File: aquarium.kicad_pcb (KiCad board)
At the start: 2 copper layers, 104 x 47 mm, 40 parts, among them U1 MOC3063, U2 MOC3063

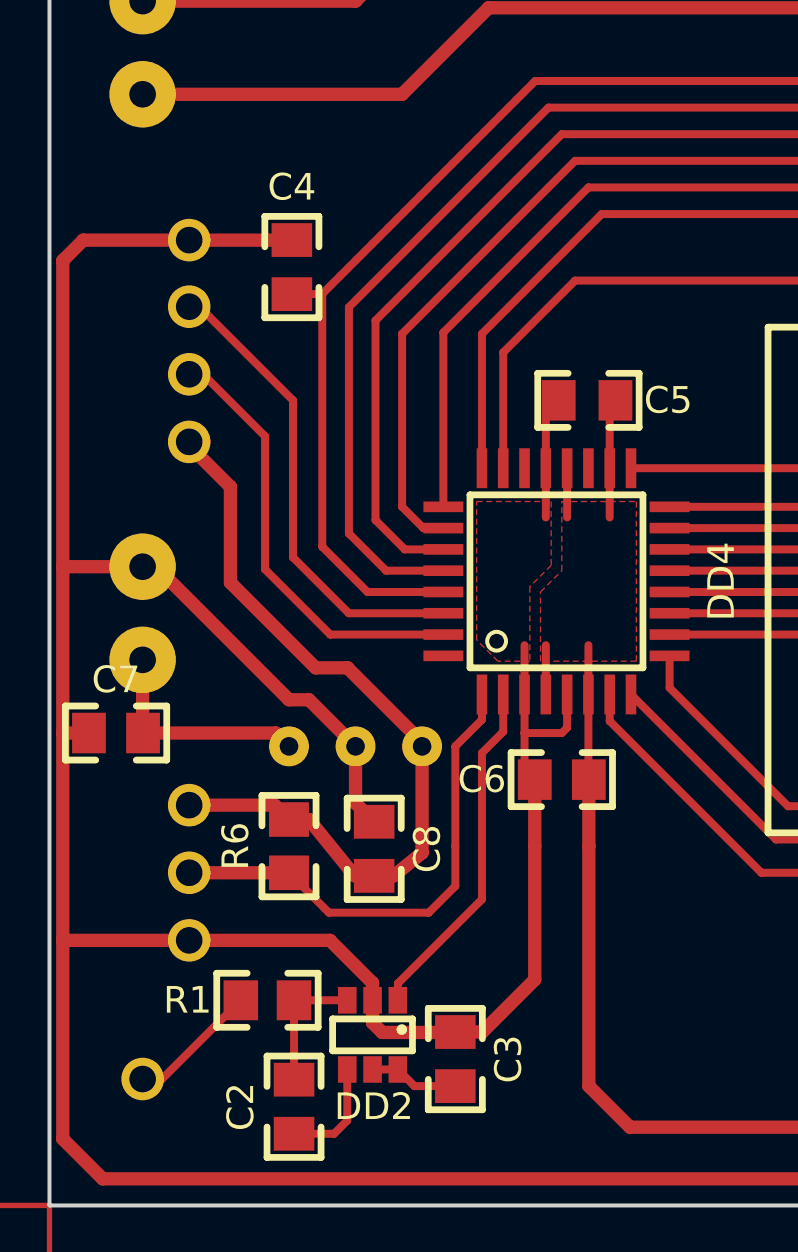
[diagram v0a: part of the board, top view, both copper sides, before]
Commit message: Revert "Added possibility to calibrate the capacitive sensor."
This reverts commit 56735a840efcf7c901892eb1b50b215983c0ef84.
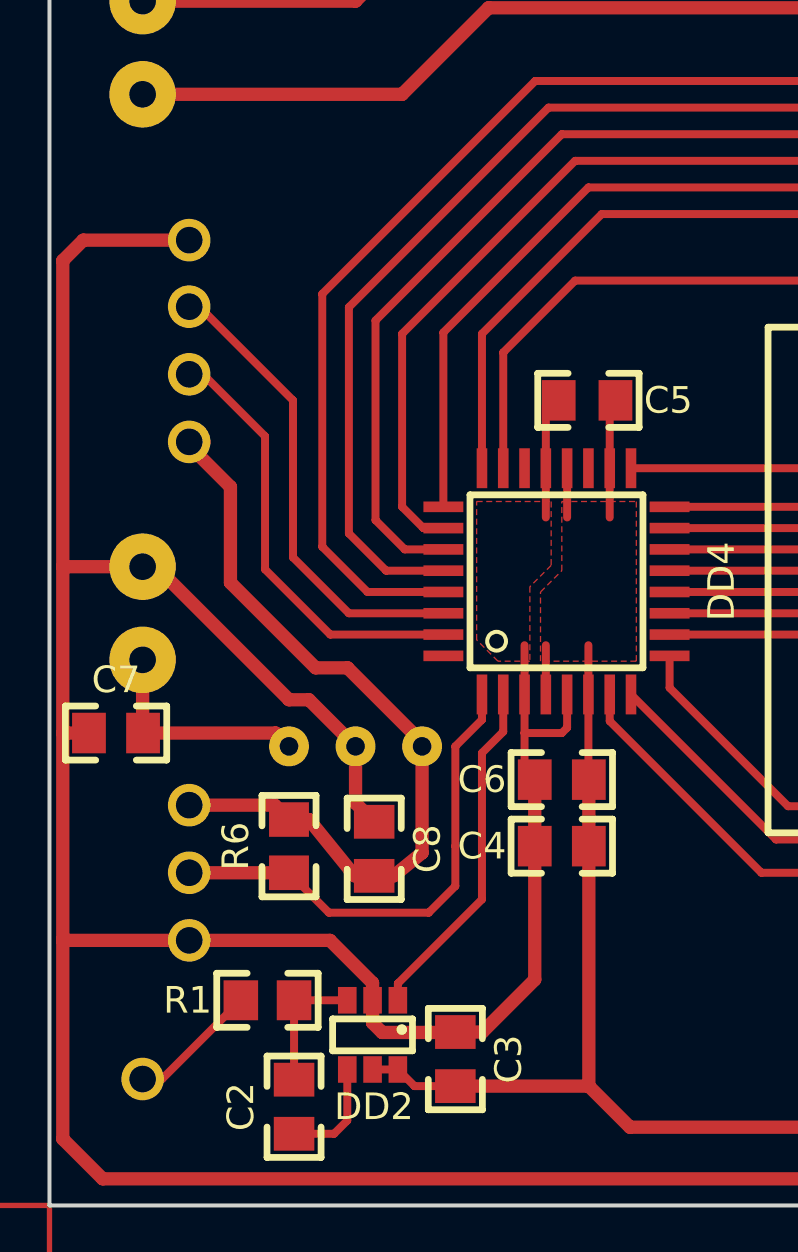
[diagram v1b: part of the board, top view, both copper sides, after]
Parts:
- moved C4 24.0 mm to (112.2, 116.5), turned to 0 degrees
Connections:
- C3 pad 1: /SENS_P -> +5B
- C4 pad 1: /~RESET -> +5B
- DD2 pad 5: /SENS_P -> +5B
- DD2 pad 6: /SENS_P -> +5B
- DD4 pad 32: /SENS_P -> Net-(DD4-Pad32)
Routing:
- net +5B: track 75.4 -> 83.9 mm
- net GND: track 248.1 -> 244.3 mm
- net /SENS_P: track 3.52 -> 0.00 mm
- net /~RESET: track 97.5 -> 96.4 mm

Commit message: Added possibility to calibrate the capacitive sensor.
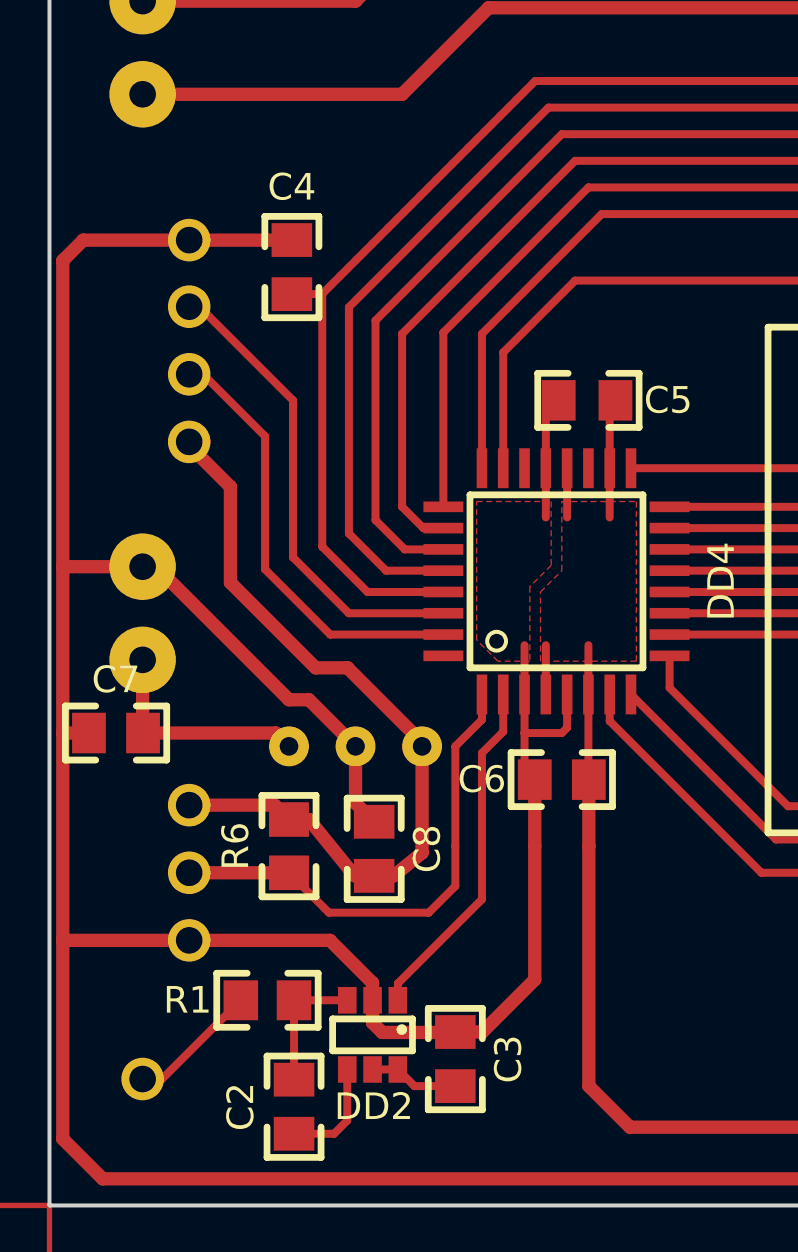
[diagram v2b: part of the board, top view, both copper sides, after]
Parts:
- moved C4 24.0 mm to (102.1, 94.7), turned to 270 degrees
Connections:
- C3 pad 1: +5B -> /SENS_P
- C4 pad 1: +5B -> /~RESET
- DD2 pad 5: +5B -> /SENS_P
- DD2 pad 6: +5B -> /SENS_P
- DD4 pad 32: Net-(DD4-Pad32) -> /SENS_P
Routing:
- net +5B: track 83.9 -> 75.4 mm
- net GND: track 244.3 -> 248.1 mm
- net /SENS_P: track 0.00 -> 3.52 mm
- net /~RESET: track 96.4 -> 97.5 mm
